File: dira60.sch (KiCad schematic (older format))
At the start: 21 parts, among them U0 ATmega32U4-AU, X0 XTAL_GND

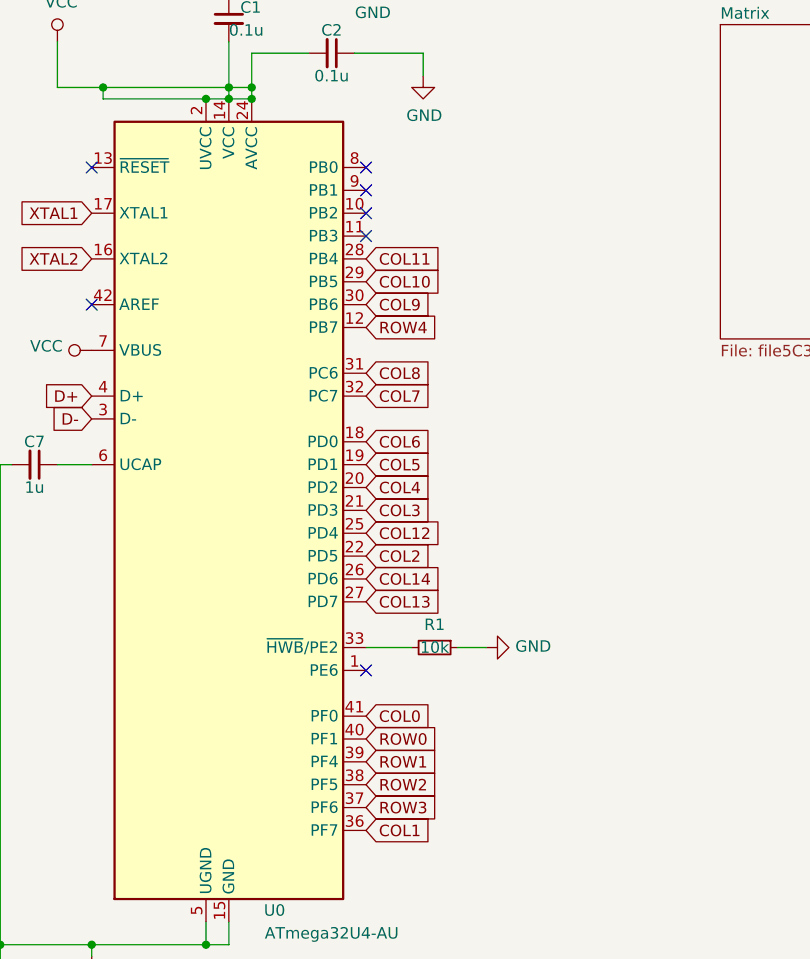
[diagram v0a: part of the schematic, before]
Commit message: Routed everything
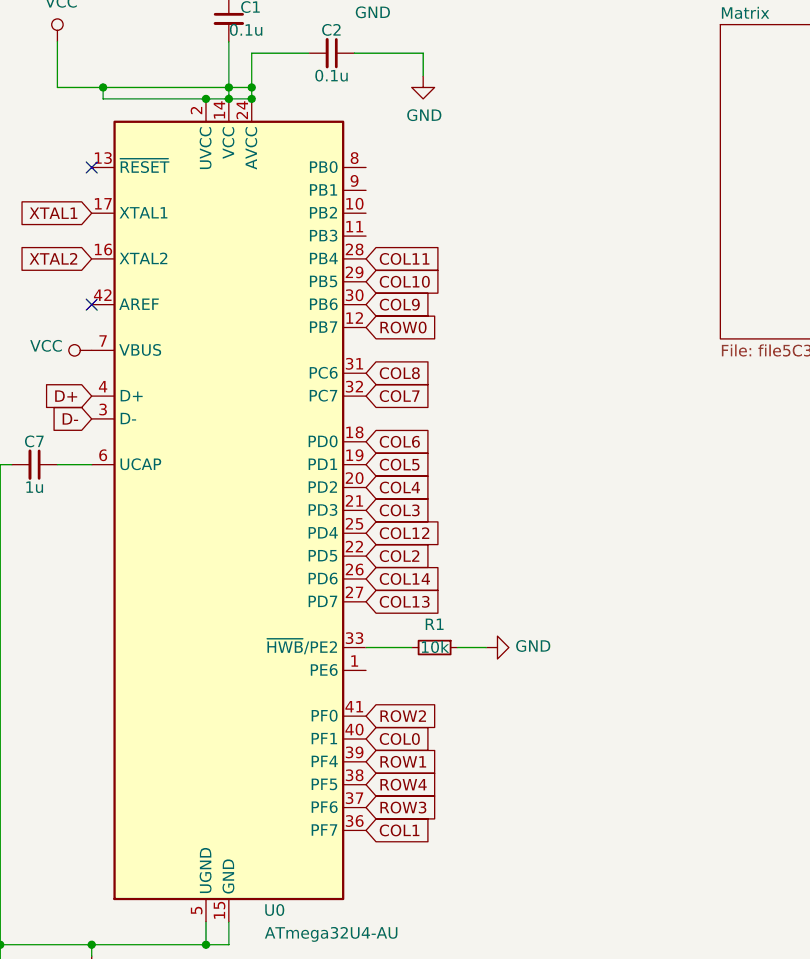
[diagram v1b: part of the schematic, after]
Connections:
- net COL0: now also U0.40 (PF1); no longer U0.41 (PF0)
- net ROW0: now also U0.12 (PB7); no longer U0.40 (PF1)
- net ROW2: now also U0.41 (PF0); no longer U0.38 (PF5)
- net ROW4: now also U0.38 (PF5); no longer U0.12 (PB7)
- no-connect marks 9 -> 4
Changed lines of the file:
@@
-$EndComp
-$Comp
-L MCU_Microchip_ATmega:ATmega32U4-AU U0
-U 1 1 5C3A488E
-P 5500 3250
-F 0 "U0" H 5700 1500 50  0000 C CNN
-F 1 "ATmega32U4-AU" H 5950 1400 50  0000 C CNN
-F 2 "keyboard_parts:QFN-44-1EP_7x7mm_Pitch0.5mm" H 5500 3250 50  0001 C CIN
-F 3 "http://ww1.microchip.com/downloads/en/DeviceDoc/Atmel-7766-8-bit-AVR-ATmega16U4-32U4_Datasheet.pdf" H 5500 3250 50  0001 C CNN
-	1    5500 3250
-	1    0    0    -1
 $EndComp
 $Comp
@@
 Text GLabel 4900 2150 0    50   Input ~ 0
 XTAL2
-Text GLabel 6100 4250 2    50   Input ~ 0
+Text GLabel 6100 2450 2    50   Input ~ 0
 ROW0
 Text GLabel 6100 4350 2    50   Input ~ 0
 ROW1
-Text GLabel 6100 4450 2    50   Input ~ 0
+Text GLabel 6100 4150 2    50   Input ~ 0
 ROW2
 Text GLabel 6100 4550 2    50   Input ~ 0
@@
 Text GLabel 6100 4650 2    50   Input ~ 0
 COL1
-Text GLabel 6100 4150 2    50   Input ~ 0
+Text GLabel 6100 4250 2    50   Input ~ 0
 COL0
 Text GLabel 6100 3650 2    50   Input ~ 0
 COL13
-Connection ~ 5400 1450
-Connection ~ 5600 1450
-Wire Wire Line
-	5400 1450 5500 1450
-Wire Wire Line
-	5400 1450 4950 1450
 Connection ~ 4500 5150
 Wire Wire Line
@@
 Wire Wire Line
 	9800 5850 10150 5850
-Text GLabel 6100 2450 2    50   Input ~ 0
+Text GLabel 6100 4450 2    50   Input ~ 0
 ROW4
-NoConn ~ 6100 3950
-NoConn ~ 6100 1950
-NoConn ~ 6100 1850
-NoConn ~ 6100 1750
-NoConn ~ 6100 2050
+Connection ~ 5600 1450
+Wire Wire Line
+	5400 1450 4950 1450
+Wire Wire Line
+	5400 1450 5500 1450
+Connection ~ 5400 1450
+$Comp
+L MCU_Microchip_ATmega:ATmega32U4-AU U0
+U 1 1 5C3A488E
+P 5500 3250
+F 0 "U0" H 5700 1500 50  0000 C CNN
+F 1 "ATmega32U4-AU" H 5950 1400 50  0000 C CNN
+F 2 "keyboard_parts:QFN-44-1EP_7x7mm_Pitch0.5mm" H 5500 3250 50  0001 C CIN
+F 3 "http://ww1.microchip.com/downloads/en/DeviceDoc/Atmel-7766-8-bit-AVR-ATmega16U4-32U4_Datasheet.pdf" H 5500 3250 50  0001 C CNN
+	1    5500 3250
+	1    0    0    -1
+$EndComp
 $EndSCHEMATC
